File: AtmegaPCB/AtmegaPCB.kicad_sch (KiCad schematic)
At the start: 175 parts, among them SW1 SW_Push, U1 PRTR5V0U2X, U2 ATmega32U4-A, Y1 16MHz

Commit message: Matrix Start
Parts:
- MX65: footprint MX_Alps_Hybrid:MX-1U-NoLED -> (none)
- MX66: footprint MX_Alps_Hybrid:MX-2.75U-NoLED -> (none)
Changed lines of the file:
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@@
       (effects (font (size 0.508 0.508)))
     )
-    (property "Footprint" "MX_Alps_Hybrid:MX-2.75U-NoLED" (id 2) (at 203.2 153.797 0)
+    (property "Footprint" "" (id 2) (at 203.2 153.797 0)
       (effects (font (size 1.524 1.524)) hide)
     )
@@
       (effects (font (size 0.508 0.508)))
     )
-    (property "Footprint" "MX_Alps_Hybrid:MX-1U-NoLED" (id 2) (at 190.373 153.797 0)
+    (property "Footprint" "" (id 2) (at 190.373 153.797 0)
       (effects (font (size 1.524 1.524)) hide)
     )
@@
     )
     (path "/e87c40d9-f420-49a1-8067-ecc2fe34d96e"
-      (reference "MX65") (unit 1) (value "MX-NoLED") (footprint "MX_Alps_Hybrid:MX-1U-NoLED")
+      (reference "MX65") (unit 1) (value "MX-NoLED") (footprint "MX_Alps_Hybrid:MX-2.75U-NoLED")
     )
     (path "/c75dd2cd-8695-4d6a-9129-fb088fec4d8f"
-      (reference "MX66") (unit 1) (value "MX-NoLED") (footprint "MX_Alps_Hybrid:MX-2.75U-NoLED")
+      (reference "MX66") (unit 1) (value "MX-NoLED") (footprint "MX_Alps_Hybrid:MX-1U-NoLED")
     )
     (path "/7e3e0cb4-b1fc-435b-bb48-b266b8669056"

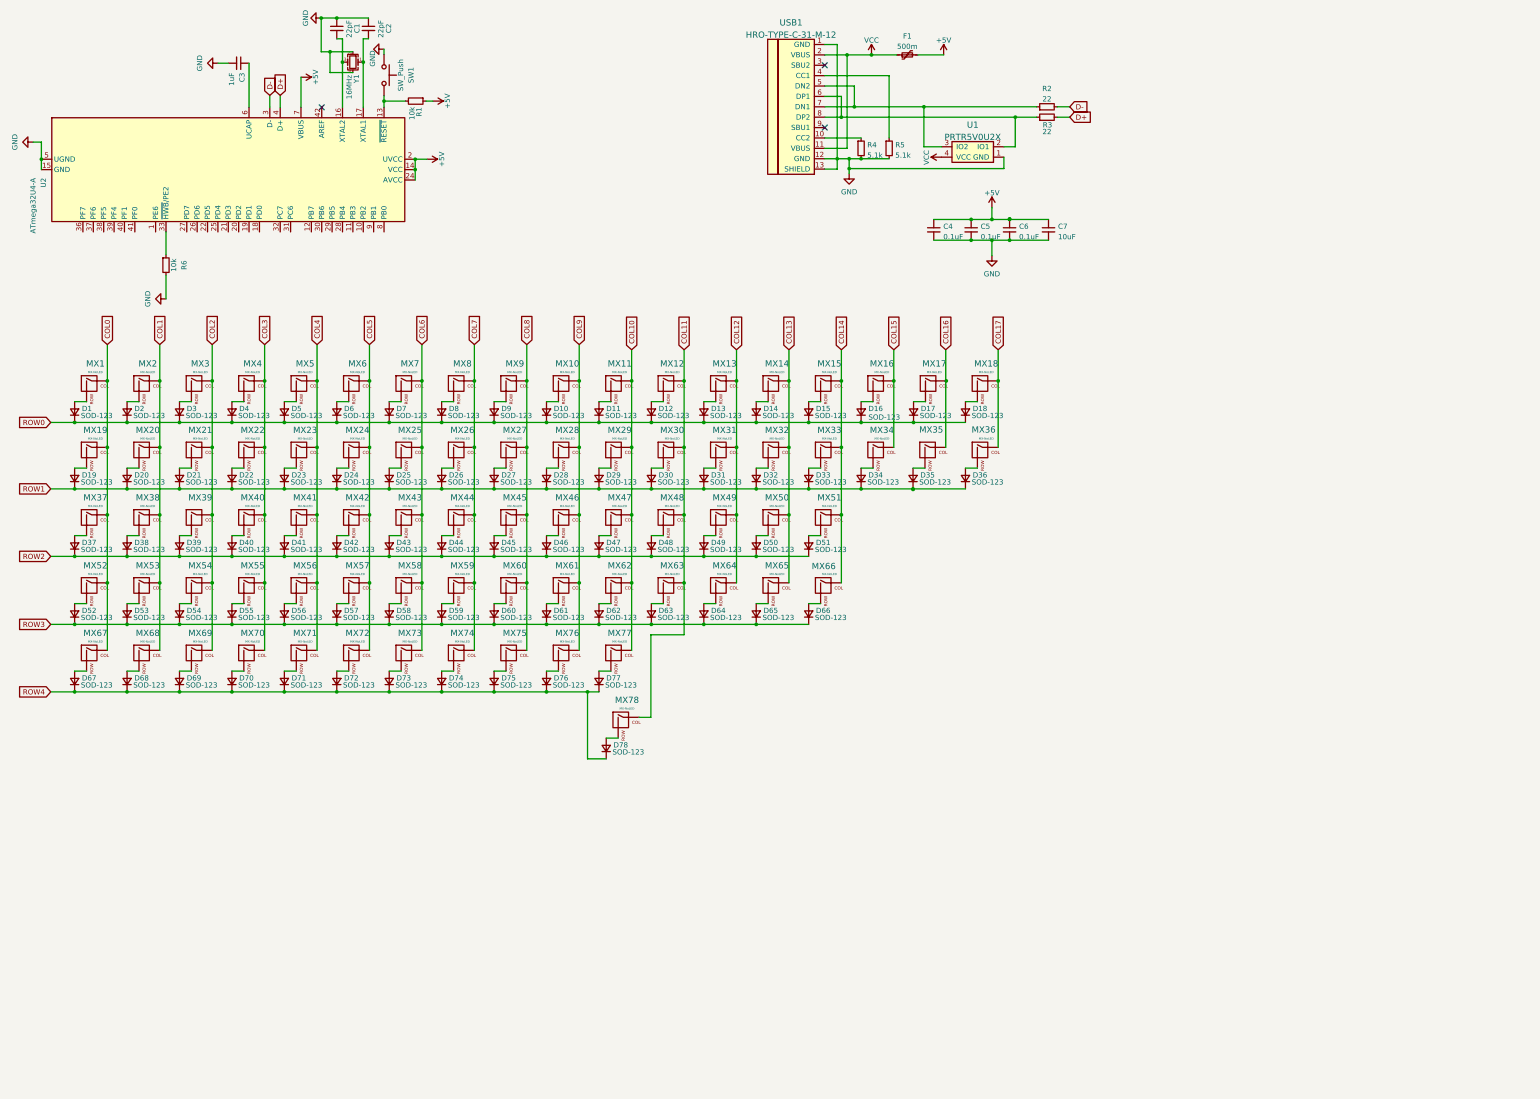
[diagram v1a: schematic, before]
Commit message: Keymap Setup
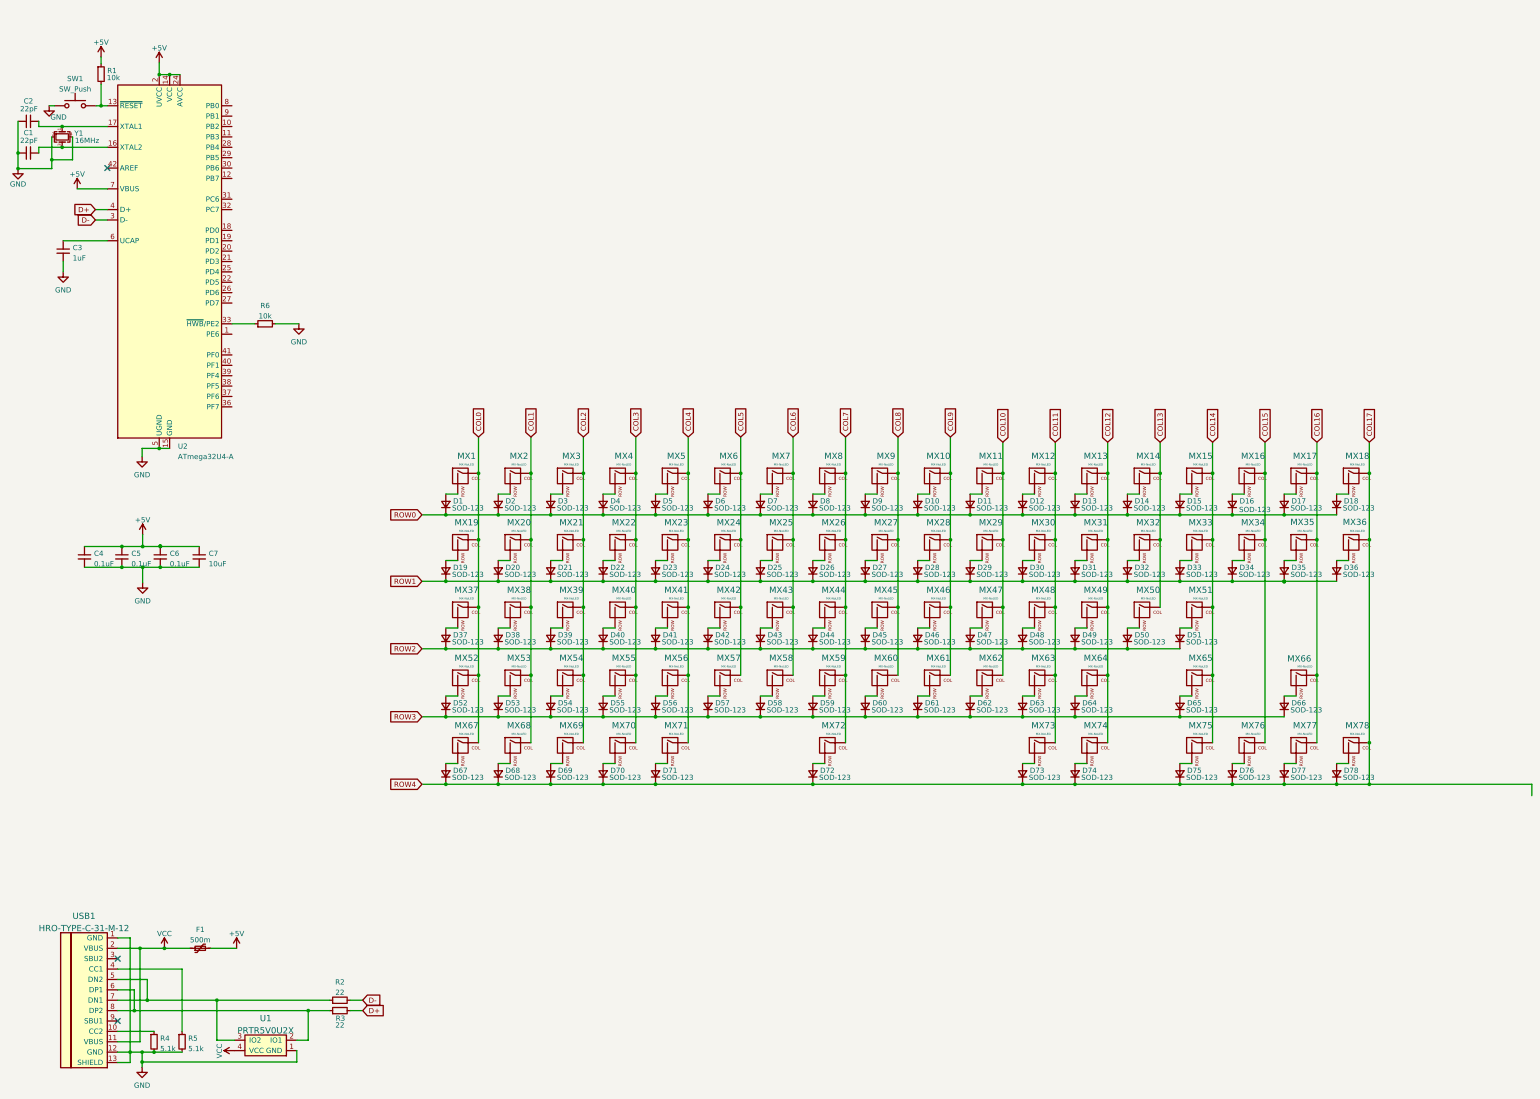
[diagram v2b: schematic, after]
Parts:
- MX21, MX34: footprint (none) -> MX_Alps_Hybrid:MX-1.5U-NoLED
- MX35: value (none) -> MX-NoLED; footprint (none) -> MX_Alps_Hybrid:MX-1U-NoLED
- MX39: value (none) -> MX-NoLED; footprint (none) -> MX_Alps_Hybrid:MX-1.75U-NoLED
- MX40, MX66: footprint (none) -> MX_Alps_Hybrid:MX-1U-NoLED
- MX51: footprint (none) -> MX_Alps_Hybrid:MX-2.25U-NoLED
- MX65: footprint (none) -> MX_Alps_Hybrid:MX-2.75U-NoLED
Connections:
- net ROW4 is gone; now on net COL17: D67.1 (K), D68.1 (K), D69.1 (K), D70.1 (K), D71.1 (K), D72.1 (K), D73.1 (K), D74.1 (K), D75.1 (K), D76.1 (K), D77.1 (K), D78.1 (K)
- net COL10: no longer MX77.1 (COL)
- net COL11: now also MX73.1 (COL); no longer MX78.1 (COL)
- net COL12: now also MX74.1 (COL)
- net COL13: no longer MX65.1 (COL)
- net COL14: now also MX65.1 (COL), MX75.1 (COL); no longer MX66.1 (COL)
- net COL15: now also MX76.1 (COL)
- net COL16: now also MX17.1 (COL), MX35.1 (COL), MX66.1 (COL), MX77.1 (COL)
- net COL17: now also MX78.1 (COL)
- net COL5: no longer MX72.1 (COL)
- net COL6: no longer MX73.1 (COL)
- net COL7: now also MX72.1 (COL); no longer MX74.1 (COL)
- net COL8: no longer MX75.1 (COL)
- net COL9: no longer MX76.1 (COL)
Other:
- moved on the sheet: C1, C2, C3, C4, C5, C6, C7, D1, D10, D11, D12, D13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
